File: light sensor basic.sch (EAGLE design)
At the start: 11 parts, among them J1 UJ2-MIBH-G-SMT-TR, U1 VCNT2020

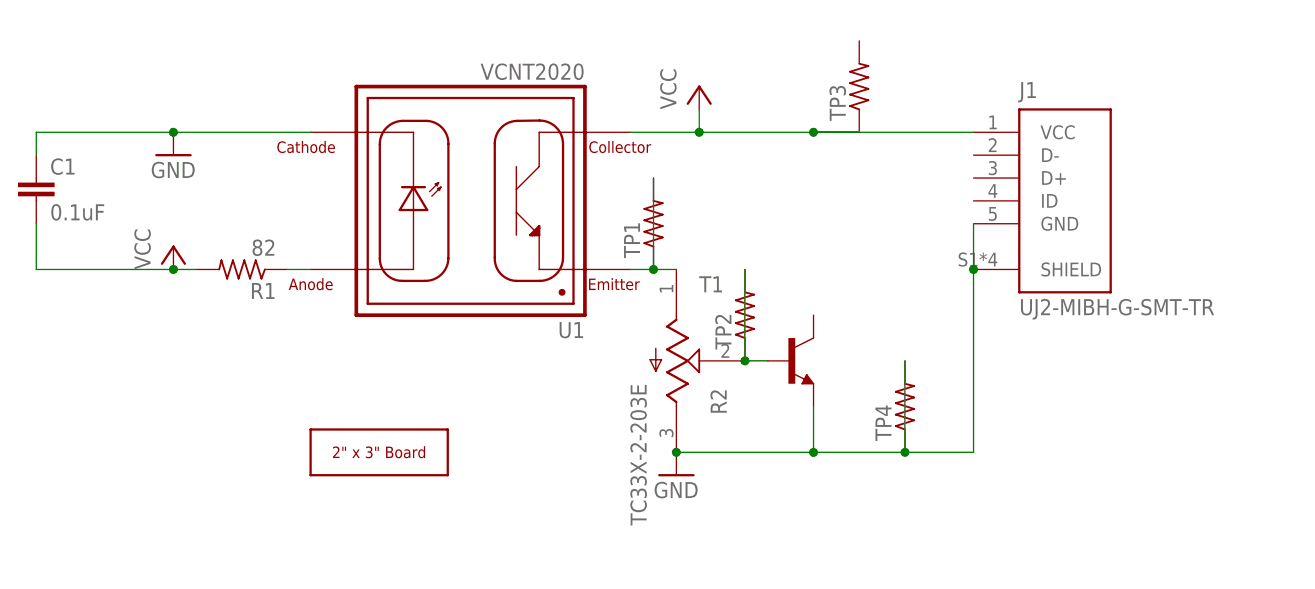
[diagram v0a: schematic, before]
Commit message: Add files via upload
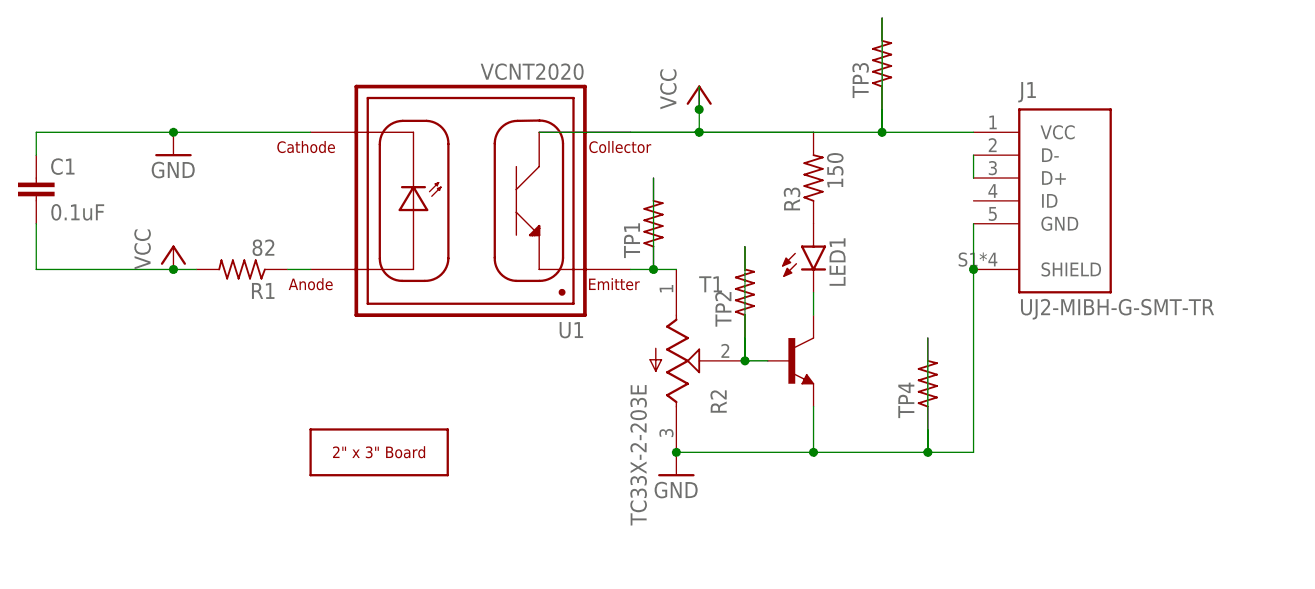
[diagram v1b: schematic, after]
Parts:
- added LED1: (no value), led:LEDSML0805
- added R3: 150, rcl:R-US_R0805
- TP1: device rcl:R-US_R1206 -> rcl:R-US_R0805
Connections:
- new net N$12: LED1.A, R3.1
- new net N$2: J1.D+, J1.D-
- new net N$5: LED1.C, T1.C
- net VCC: now also R3.2, TP3.2
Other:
- moved on the sheet: TP2, TP3, TP4
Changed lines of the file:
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@@
 <part name="TP3" library="rcl" library_urn="urn:adsk.eagle:library:334" deviceset="R-US_" device="R1206" package3d_urn="urn:adsk.eagle:package:23540/2"/>
 <part name="TP4" library="rcl" library_urn="urn:adsk.eagle:library:334" deviceset="R-US_" device="R1206" package3d_urn="urn:adsk.eagle:package:23540/2"/>
-<part name="TP1" library="rcl" library_urn="urn:adsk.eagle:library:334" deviceset="R-US_" device="R1206" package3d_urn="urn:adsk.eagle:package:23540/2"/>
 <part name="TP2" library="rcl" library_urn="urn:adsk.eagle:library:334" deviceset="R-US_" device="R1206" package3d_urn="urn:adsk.eagle:package:23540/2"/>
+<part name="LED1" library="led" library_urn="urn:adsk.eagle:library:259" deviceset="LED" device="SML0805" package3d_urn="urn:adsk.eagle:package:15830/1"/>
+<part name="R3" library="rcl" library_urn="urn:adsk.eagle:library:334" deviceset="R-US_" device="R0805" package3d_urn="urn:adsk.eagle:package:23553/2" value="150"/>
+<part name="TP1" library="rcl" library_urn="urn:adsk.eagle:library:334" deviceset="R-US_" device="R0805" package3d_urn="urn:adsk.eagle:package:23553/2"/>
 </parts>
 <sheets>
@@
 <attribute name="VALUE" x="96.52" y="40.64" size="1.778" layer="96"/>
 </instance>
-<instance part="TP3" gate="G$1" x="78.74" y="66.04" smashed="yes" rot="R90">
-<attribute name="NAME" x="77.2414" y="62.23" size="1.778" layer="95" rot="R90"/>
-<attribute name="VALUE" x="82.042" y="62.23" size="1.778" layer="96" rot="R90"/>
+<instance part="TP3" gate="G$1" x="81.28" y="68.58" smashed="yes" rot="R90">
+<attribute name="NAME" x="79.7814" y="64.77" size="1.778" layer="95" rot="R90"/>
+<attribute name="VALUE" x="84.582" y="64.77" size="1.778" layer="96" rot="R90"/>
 </instance>
-<instance part="TP4" gate="G$1" x="83.82" y="30.48" smashed="yes" rot="R90">
-<attribute name="NAME" x="82.3214" y="26.67" size="1.778" layer="95" rot="R90"/>
-<attribute name="VALUE" x="87.122" y="26.67" size="1.778" layer="96" rot="R90"/>
+<instance part="TP4" gate="G$1" x="86.36" y="33.02" smashed="yes" rot="R90">
+<attribute name="NAME" x="84.8614" y="29.21" size="1.778" layer="95" rot="R90"/>
+<attribute name="VALUE" x="89.662" y="29.21" size="1.778" layer="96" rot="R90"/>
+</instance>
+<instance part="TP2" gate="G$1" x="66.04" y="43.18" smashed="yes" rot="R90">
+<attribute name="NAME" x="64.5414" y="39.37" size="1.778" layer="95" rot="R90"/>
+<attribute name="VALUE" x="69.342" y="39.37" size="1.778" layer="96" rot="R90"/>
+</instance>
+<instance part="LED1" gate="G$1" x="73.66" y="48.26" smashed="yes">
+<attribute name="NAME" x="77.216" y="43.688" size="1.778" layer="95" rot="R90"/>
+<attribute name="VALUE" x="79.375" y="43.688" size="1.778" layer="96" rot="R90"/>
+</instance>
+<instance part="R3" gate="G$1" x="73.66" y="55.88" smashed="yes" rot="R90">
+<attribute name="NAME" x="72.1614" y="52.07" size="1.778" layer="95" rot="R90"/>
+<attribute name="VALUE" x="76.962" y="54.61" size="1.778" layer="96" rot="R90"/>
 </instance>
 <instance part="TP1" gate="G$1" x="55.88" y="50.8" smashed="yes" rot="R90">
 <attribute name="NAME" x="54.3814" y="46.99" size="1.778" layer="95" rot="R90"/>
 <attribute name="VALUE" x="59.182" y="46.99" size="1.778" layer="96" rot="R90"/>
-</instance>
-<instance part="TP2" gate="G$1" x="66.04" y="40.64" smashed="yes" rot="R90">
-<attribute name="NAME" x="64.5414" y="36.83" size="1.778" layer="95" rot="R90"/>
-<attribute name="VALUE" x="69.342" y="36.83" size="1.778" layer="96" rot="R90"/>
 </instance>
 </instances>
@@
 <pinref part="R1" gate="G$1" pin="2"/>
 <pinref part="P+1" gate="VCC" pin="VCC"/>
-<wire x1="5.08" y1="45.72" x2="2.54" y2="45.72" width="0.1524" layer="91"/>
 <pinref part="C1" gate="G$1" pin="2"/>
 <wire x1="-12.7" y1="50.8" x2="-12.7" y2="45.72" width="0.1524" layer="91"/>
 <wire x1="-12.7" y1="45.72" x2="2.54" y2="45.72" width="0.1524" layer="91"/>
 <junction x="2.54" y="45.72"/>
+<wire x1="2.54" y1="45.72" x2="5.08" y2="45.72" width="0.1524" layer="91"/>
 </segment>
 <segment>
@@
 <pinref part="P+2" gate="VCC" pin="VCC"/>
 <wire x1="60.96" y1="60.96" x2="60.96" y2="63.5" width="0.1524" layer="91"/>
+<junction x="60.96" y="60.96"/>
+<pinref part="R3" gate="G$1" pin="2"/>
 <wire x1="60.96" y1="60.96" x2="73.66" y2="60.96" width="0.1524" layer="91"/>
-<junction x="60.96" y="60.96"/>
+<wire x1="60.96" y1="63.5" x2="60.96" y2="66.04" width="0.1524" layer="91"/>
+<junction x="60.96" y="63.5"/>
+<wire x1="60.96" y1="60.96" x2="43.18" y2="60.96" width="0.1524" layer="91"/>
 <pinref part="J1" gate="G$1" pin="VCC"/>
+<wire x1="60.96" y1="60.96" x2="81.28" y2="60.96" width="0.1524" layer="91"/>
 <pinref part="TP3" gate="G$1" pin="1"/>
-<wire x1="73.66" y1="60.96" x2="91.44" y2="60.96" width="0.1524" layer="91"/>
-<junction x="73.66" y="60.96"/>
-<wire x1="73.66" y1="60.96" x2="78.74" y2="60.96" width="0.1524" layer="91"/>
+<wire x1="81.28" y1="60.96" x2="91.44" y2="60.96" width="0.1524" layer="91"/>
+<wire x1="81.28" y1="63.5" x2="81.28" y2="60.96" width="0.1524" layer="91"/>
+<junction x="81.28" y="60.96"/>
+<pinref part="TP3" gate="G$1" pin="2"/>
+<wire x1="81.28" y1="73.66" x2="81.28" y2="60.96" width="0.1524" layer="91"/>
 </segment>
 </net>
@@
 </segment>
 <segment>
+<pinref part="T1" gate="G$1" pin="E"/>
+<wire x1="73.66" y1="25.4" x2="73.66" y2="30.48" width="0.1524" layer="91"/>
 <pinref part="R2" gate="G$1" pin="CW"/>
 <pinref part="GND2" gate="1" pin="GND"/>
 <wire x1="58.42" y1="25.4" x2="73.66" y2="25.4" width="0.1524" layer="91"/>
 <junction x="58.42" y="25.4"/>
-<pinref part="T1" gate="G$1" pin="E"/>
-<wire x1="73.66" y1="25.4" x2="73.66" y2="30.48" width="0.1524" layer="91"/>
+<wire x1="73.66" y1="25.4" x2="86.36" y2="25.4" width="0.1524" layer="91"/>
+<junction x="73.66" y="25.4"/>
+<pinref part="TP4" gate="G$1" pin="1"/>
+<wire x1="86.36" y1="25.4" x2="91.44" y2="25.4" width="0.1524" layer="91"/>
+<wire x1="86.36" y1="27.94" x2="86.36" y2="25.4" width="0.1524" layer="91"/>
+<junction x="86.36" y="25.4"/>
+<pinref part="TP4" gate="G$1" pin="2"/>
+<wire x1="86.36" y1="38.1" x2="86.36" y2="25.4" width="0.1524" layer="91"/>
 <pinref part="J1" gate="G$1" pin="GND"/>
 <pinref part="J1" gate="G$1" pin="SHIELD"/>
-<wire x1="91.44" y1="50.8" x2="91.44" y2="45.72" width="0.1524" layer="91"/>
-<wire x1="91.44" y1="25.4" x2="91.44" y2="45.72" width="0.1524" layer="91"/>
+<wire x1="91.44" y1="45.72" x2="91.44" y2="50.8" width="0.1524" layer="91"/>
+<wire x1="91.44" y1="45.72" x2="91.44" y2="25.4" width="0.1524" layer="91"/>
 <junction x="91.44" y="45.72"/>
-<wire x1="73.66" y1="25.4" x2="83.82" y2="25.4" width="0.1524" layer="91"/>
-<junction x="73.66" y="25.4"/>
-<pinref part="TP4" gate="G$1" pin="1"/>
-<wire x1="83.82" y1="25.4" x2="91.44" y2="25.4" width="0.1524" layer="91"/>
-<junction x="83.82" y="25.4"/>
-<pinref part="TP4" gate="G$1" pin="2"/>
-<wire x1="83.82" y1="35.56" x2="83.82" y2="25.4" width="0.1524" layer="91"/>
 </segment>
 </net>
-<net name="N$2" class="0">
+<net name="N$5" class="0">
+<segment>
+<pinref part="LED1" gate="G$1" pin="C"/>
+<pinref part="T1" gate="G$1" pin="C"/>
+<wire x1="73.66" y1="43.18" x2="73.66" y2="40.64" width="0.1524" layer="91"/>
+</segment>
+</net>
+<net name="N$10" class="0">
 <segment>
 <pinref part="U1" gate="VCNT2020" pin="EMITTER"/>
@@
 </segment>
 </net>
-<net name="N$3" class="0">
+<net name="N$2" class="0">
 <segment>
+<pinref part="J1" gate="G$1" pin="D-"/>
+<wire x1="91.44" y1="58.42" x2="91.44" y2="55.88" width="0.1524" layer="91"/>
+<pinref part="J1" gate="G$1" pin="D+"/>
+</segment>
+</net>
+<net name="N$12" class="0">
+<segment>
+<pinref part="R3" gate="G$1" pin="1"/>
+<pinref part="LED1" gate="G$1" pin="A"/>
+</segment>
+</net>
+<net name="N$4" class="0">
+<segment>
+<pinref part="T1" gate="G$1" pin="B"/>
 <pinref part="R2" gate="G$1" pin="W"/>
-<pinref part="T1" gate="G$1" pin="B"/>
 <wire x1="66.04" y1="35.56" x2="68.58" y2="35.56" width="0.1524" layer="91"/>
 <pinref part="TP2" gate="G$1" pin="1"/>
+<wire x1="66.04" y1="38.1" x2="66.04" y2="35.56" width="0.1524" layer="91"/>
 <junction x="66.04" y="35.56"/>
 <pinref part="TP2" gate="G$1" pin="2"/>
-<wire x1="66.04" y1="45.72" x2="66.04" y2="35.56" width="0.1524" layer="91"/>
+<wire x1="66.04" y1="48.26" x2="66.04" y2="35.56" width="0.1524" layer="91"/>
 </segment>
 </net>
